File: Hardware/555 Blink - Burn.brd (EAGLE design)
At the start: 100 x 80 mm, 80 parts, among them IC1 LM555N, IC2 LM555N, IC3 LM555N, IC4 LM555N, IC5 LM555N, IC6 LM555N, IC7 LM555N, IC8 LM555N

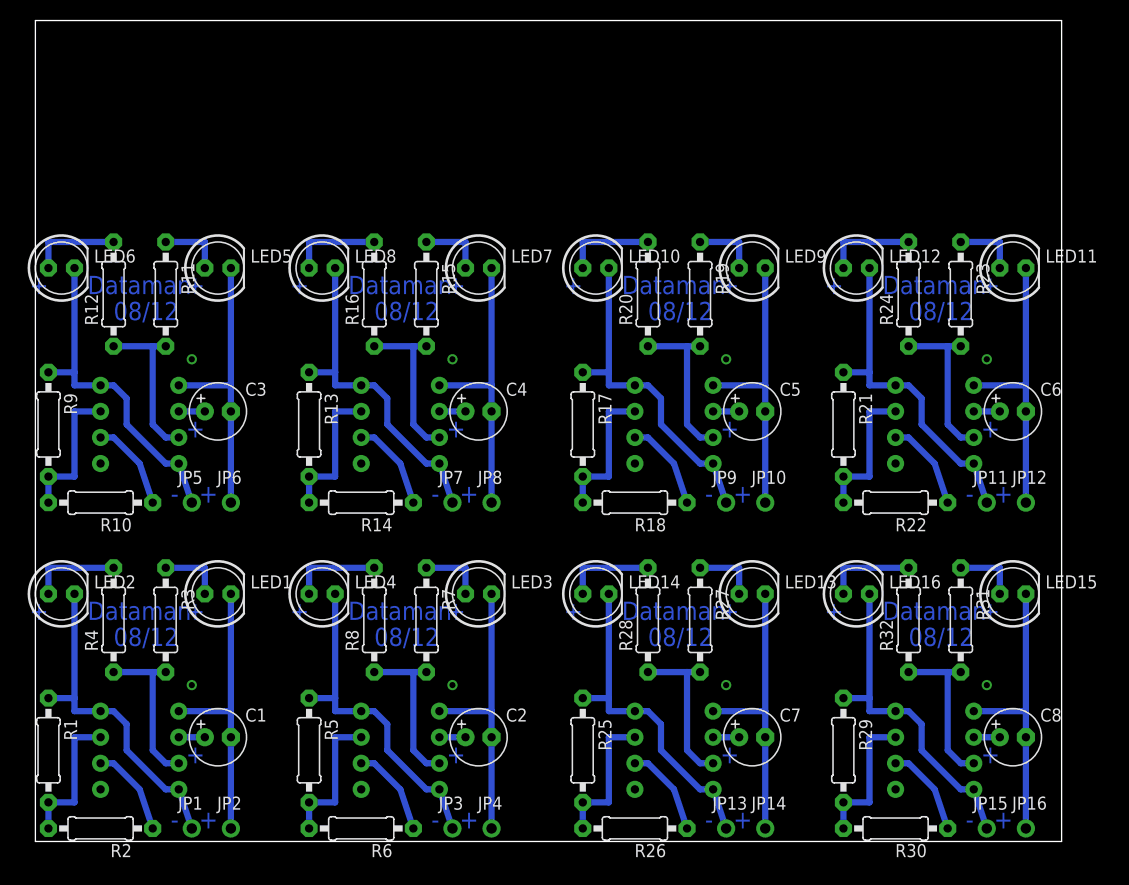
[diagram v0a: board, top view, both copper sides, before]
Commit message: Burn board for mods
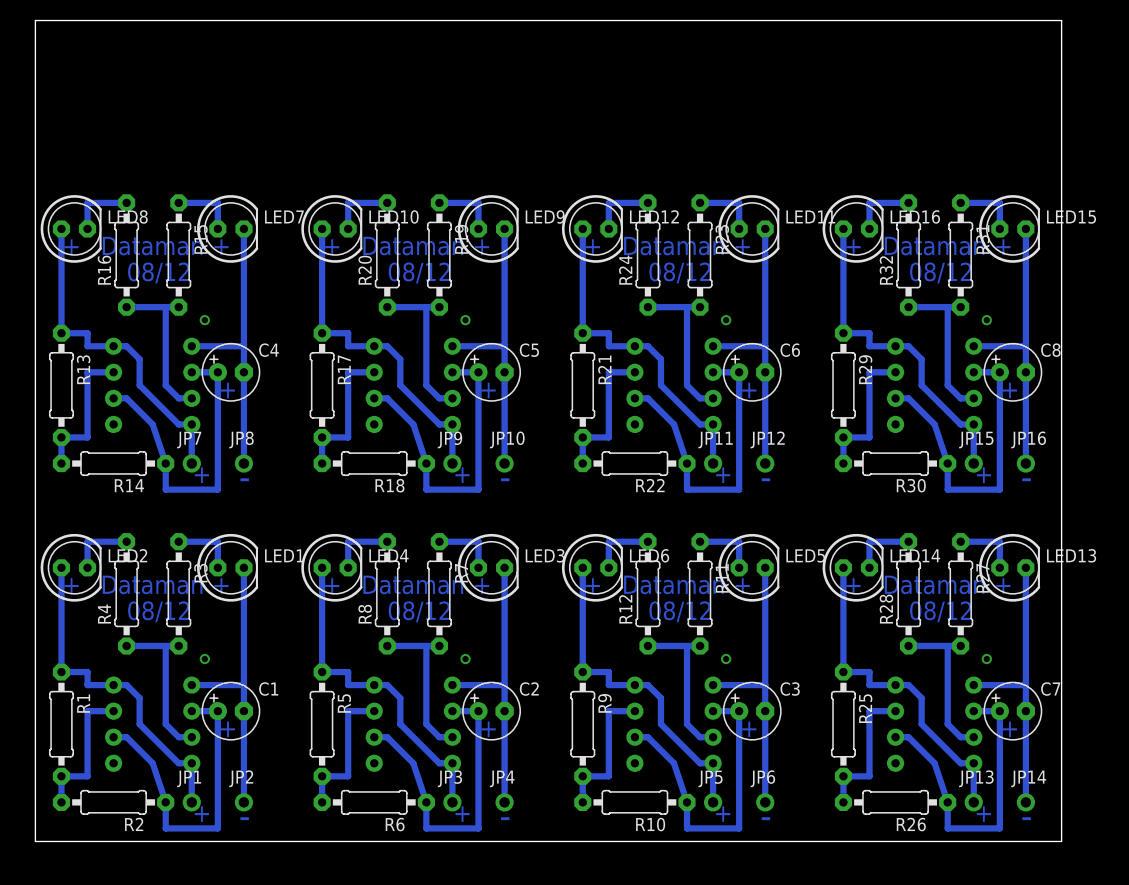
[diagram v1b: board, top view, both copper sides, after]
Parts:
- moved JP6 59.7 mm to (71.1, 3.81)
- moved R11 59.7 mm to (64.8, 24.1)
- moved LED6 59.7 mm to (54.6, 26.7)
- moved R10 59.7 mm to (58.4, 3.81)
- moved R12 59.7 mm to (59.7, 24.1)
- moved R9 59.7 mm to (53.3, 11.4)
- moved C3 59.7 mm to (69.8, 12.7)
- moved IC3 59.7 mm to (62.2, 11.4)
- moved LED5 59.7 mm to (69.8, 26.7)
- moved JP5 58.6 mm to (66.0, 3.81)
- moved JP15 35.6 mm to (91.4, 36.8)
- moved C8 35.6 mm to (95.2, 45.7)
- moved IC8 35.6 mm to (87.6, 44.5)
- moved LED15 35.6 mm to (95.2, 59.7)
- moved LED16 35.6 mm to (80.0, 59.7)
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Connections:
- removed net N$13 (its old number): LED4.A, R8.2
- removed net N$17 (its old number): C3.+, IC3.2
- removed net N$22 (its old number): IC4.6, R14.1
- removed net N$27 (its old number): LED8.A, R16.2
- removed net N$31 (its old number): C5.+, IC5.2
- removed net N$36 (its old number): IC6.6, R22.1
- removed net N$38 (its old number): C6.+, IC6.2
- removed net N$41: LED12.A, R24.2
- removed net N$43: IC7.6, R26.1
- removed net N$45: C7.+, IC7.2
- removed net N$48: LED14.A, R28.2
- removed net N$5 (its old number): C1.+, IC1.2
- removed net N$50: IC8.6, R30.1
- removed net N$52: C8.+, IC8.2
- removed net N$55: LED16.A, R32.2
- removed net N$7 (its old number): LED2.A, R4.2
- removed net N$8 (its old number): IC2.6, R6.1
- new net N$14: LED6.K, R12.2
- new net N$19: LED8.K, R16.2
- new net N$25: C5.+, IC5.2, IC5.6, R18.1
- new net N$30: C6.+, IC6.2, IC6.6, R22.1
- new net N$35: C7.+, IC7.2, IC7.6, R26.1
- new net N$39: LED16.K, R32.2
- new net N$4: LED2.K, R4.2
- new net N$40: C8.+, IC8.2, IC8.6, R30.1
- new net N$9: LED4.K, R8.2
- net +9V: now also LED2.A; no longer LED2.K
- net +9V1: now also LED4.A; no longer LED4.K
- net +9V2: now also LED6.A; no longer LED6.K
- net +9V3: now also LED8.A; no longer LED8.K
- net +9V4: now also LED10.A; no longer LED10.K
- net +9V5: now also LED12.A; no longer LED12.K
- net +9V6: now also LED14.A; no longer LED14.K
- net +9V7: now also LED16.A; no longer LED16.K
- net N$10: now also IC2.6, R6.1
- net N$15: now also C3.+, IC3.2
- net N$2: now also C1.+, IC1.2
- net N$20: now also C4.+, IC4.2, IC4.6, R14.1; no longer LED6.A, R12.2
- net N$24: now also LED10.K, R20.2; no longer C4.+, IC4.2
- net N$29: now also LED12.K, R24.2; no longer IC5.6, R18.1
- net N$34: now also LED14.K, R28.2; no longer LED10.A, R20.2
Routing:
- net N$40: track 0.00 -> 30.5 mm
- net N$35: track 0.00 -> 30.5 mm, vias 1 -> 0
- net N$25: track 0.00 -> 30.5 mm
- net N$30: track 0.00 -> 30.5 mm
- net N$10: track 2.54 -> 30.5 mm
- net N$2: track 8.88 -> 30.5 mm
- net N$15: track 8.88 -> 30.5 mm
- net N$20: track 8.89 -> 30.5 mm
- net N$55: track 8.89 -> 0.00 mm
- net N$41: track 8.89 -> 0.00 mm
- net N$13 (its old number): track 8.89 -> 0.00 mm
- net N$7 (its old number): track 8.89 -> 0.00 mm
- net N$27 (its old number): track 8.89 -> 0.00 mm
- net N$48: track 8.89 -> 0.00 mm
- net N$50: track 8.88 -> 0.00 mm
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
